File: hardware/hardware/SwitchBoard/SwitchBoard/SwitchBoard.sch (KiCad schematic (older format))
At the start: 32 parts

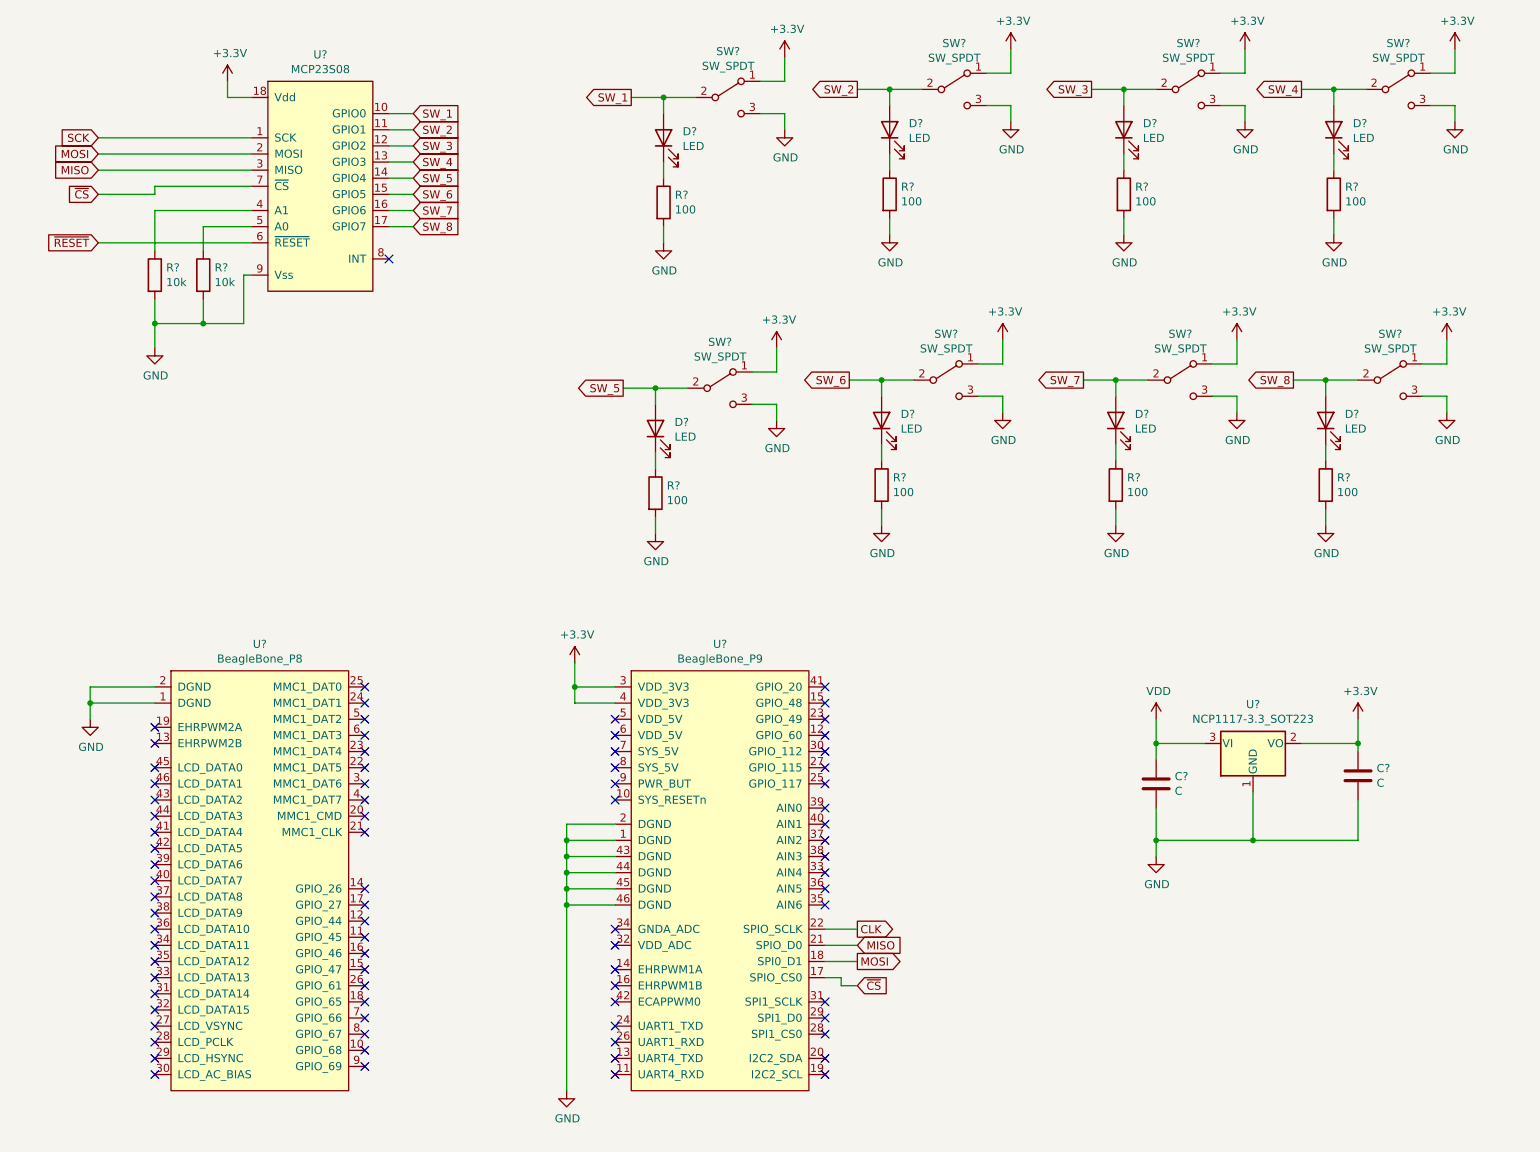
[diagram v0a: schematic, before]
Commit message: Finished Switchboard schematic and BOM
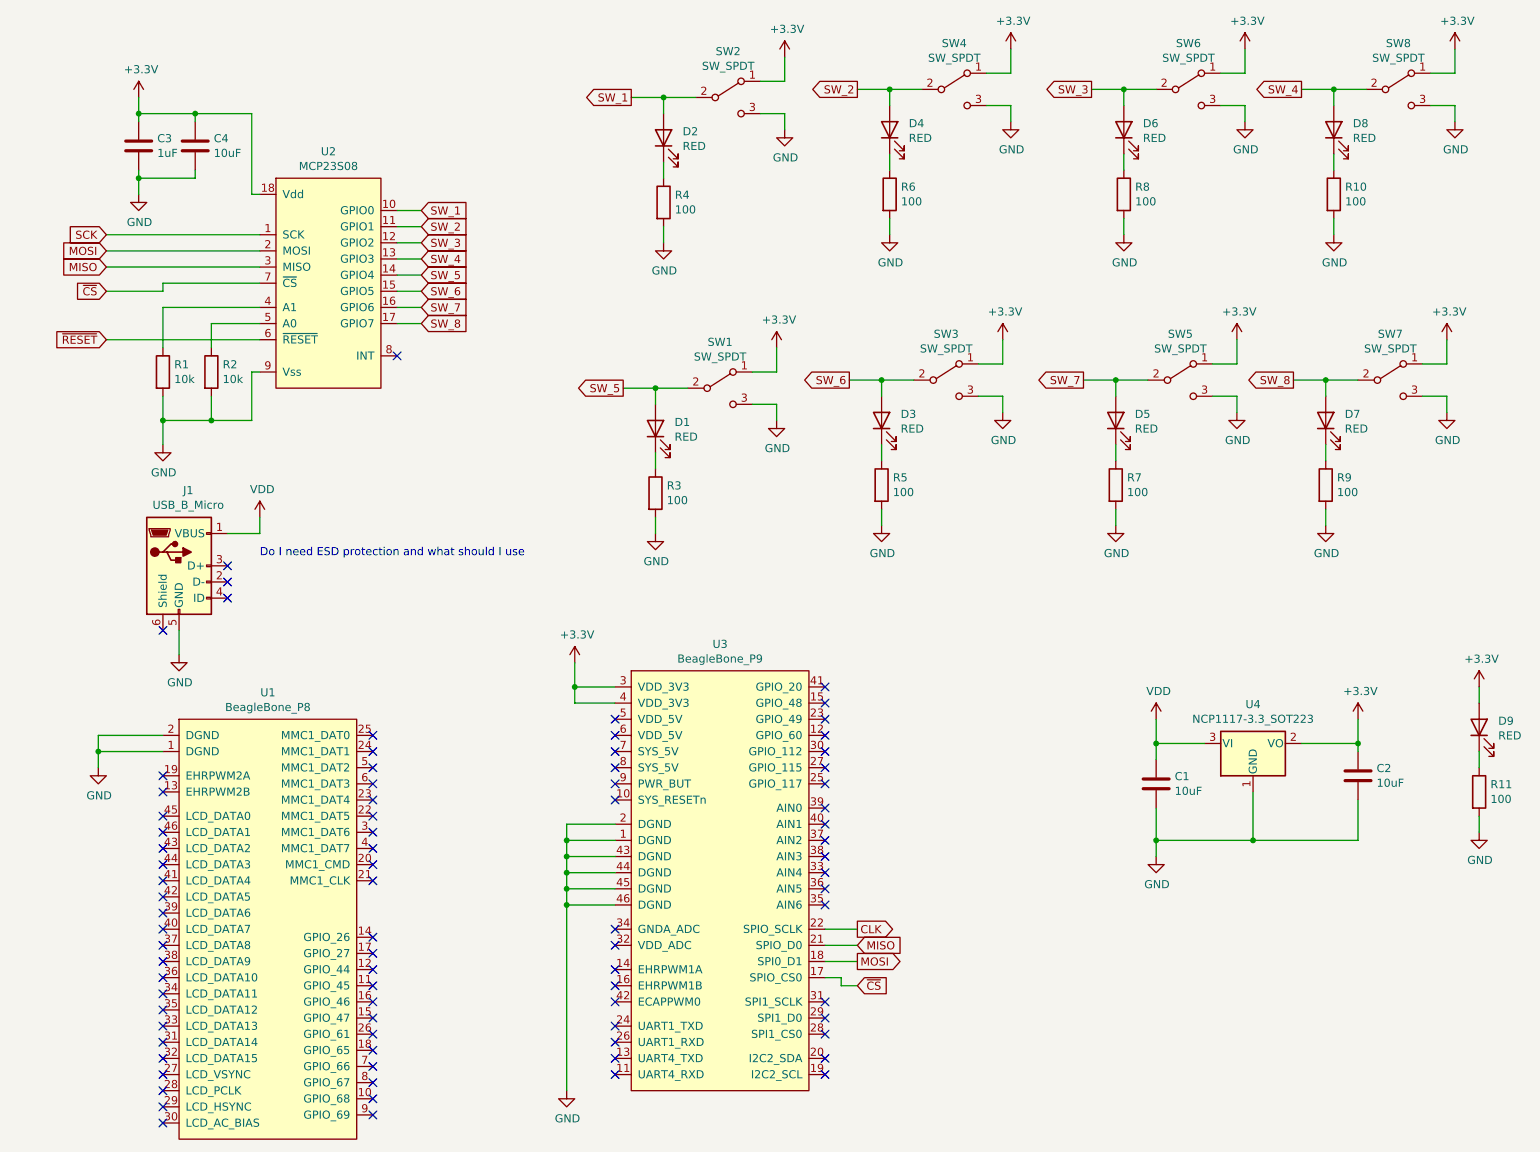
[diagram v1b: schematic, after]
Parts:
- added C3: 1uF, symbol Device:C
- added C4: 10uF, symbol Device:C
- added D9: RED, symbol Device:LED
- added J1: USB_B_Micro, symbol Connector:USB_B_Micro
- added R11: 100, symbol Device:R
- C1, C2: renamed from C?; value C -> 10uF; Digikey Part Number (none) -> 1276-1038-1-ND
- D1, D2, D3, D4, D5, D6, D7, D8: renamed from D?; value LED -> RED; Digikey Part Number (none) -> 732-4978-1-ND
- R1, R2: renamed from R?; Digikey Part Number (none) -> 13-RT0603FRE1310KLCT-ND
- R10, R3, R4, R5, R6, R7, R8, R9: renamed from R?; Digikey Part Number (none) -> 118-CR0603AFX-1000ELFCT-ND
- SW1, SW2, SW3, SW4, SW5, SW6, SW7, SW8: renamed from SW?; Digikey Part Number (none) -> 401-2002-1-ND
- U1: renamed from U?; Digikey Part Number (none) -> 1528-1365-ND
- U2: renamed from U?; Digikey Part Number (none) -> MCP23S08-E/SO-ND
- U3: renamed from U?; Digikey Part Number (none) -> NA
- U4: renamed from U?; Digikey Part Number (none) -> 488-NCP1117IST33T3GCT-ND
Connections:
- net +3V3: now also C3.1, C4.1, D9.2 (A)
- net GND: now also C3.2, C4.2, J1.5 (GND), R11.2
- net VDD: now also J1.1 (VBUS)
- new net: D9.1 (K), R11.1
- no-connect marks 79 -> 83
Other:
- note added: "Do I need ESD protection and what should I use"
- moved on the sheet: R1, R2, U1, U2
